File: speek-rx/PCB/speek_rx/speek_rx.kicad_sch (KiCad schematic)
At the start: 69 parts, among them CN1 PJ-320D, CN2 PJ-320D, J1 Conn_01x02, J3 Conn_01x06_Socket, J4 Conn_01x04, U1 ESP32-D0WD-V3, U2 W25Q32JVSSIQ_C179173, U3 CP2102N-A02-GQFN24R, U4 SPX1117M3-L-3-3/TR, U5 PCM5102APW, U6 TPA6132A2RTER, X1 XL2EL89CPI-111YLC-40M

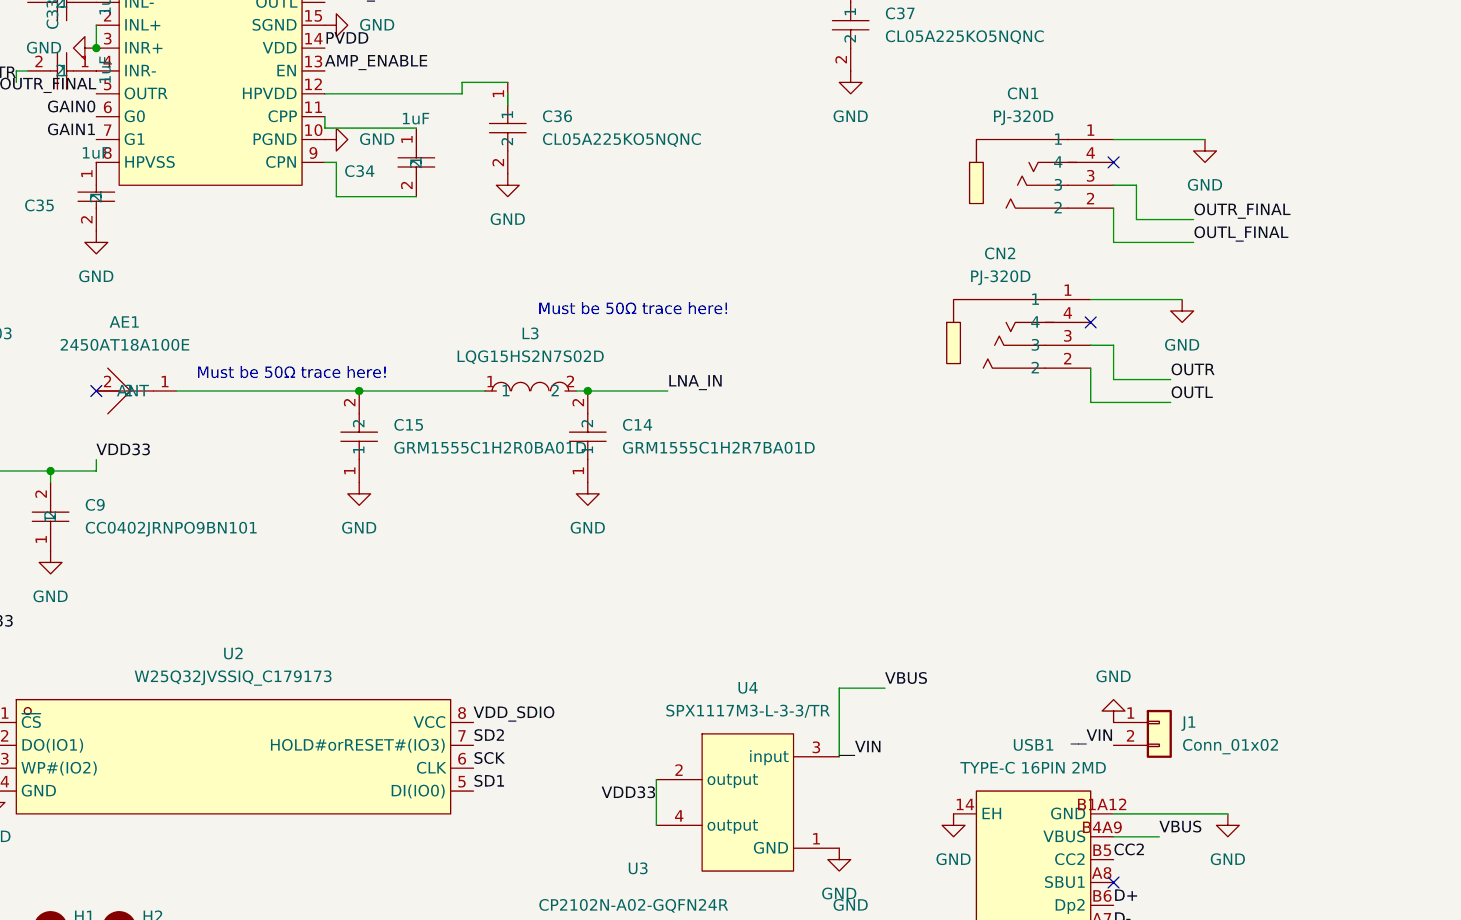
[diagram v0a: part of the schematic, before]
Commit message: JST and antenna
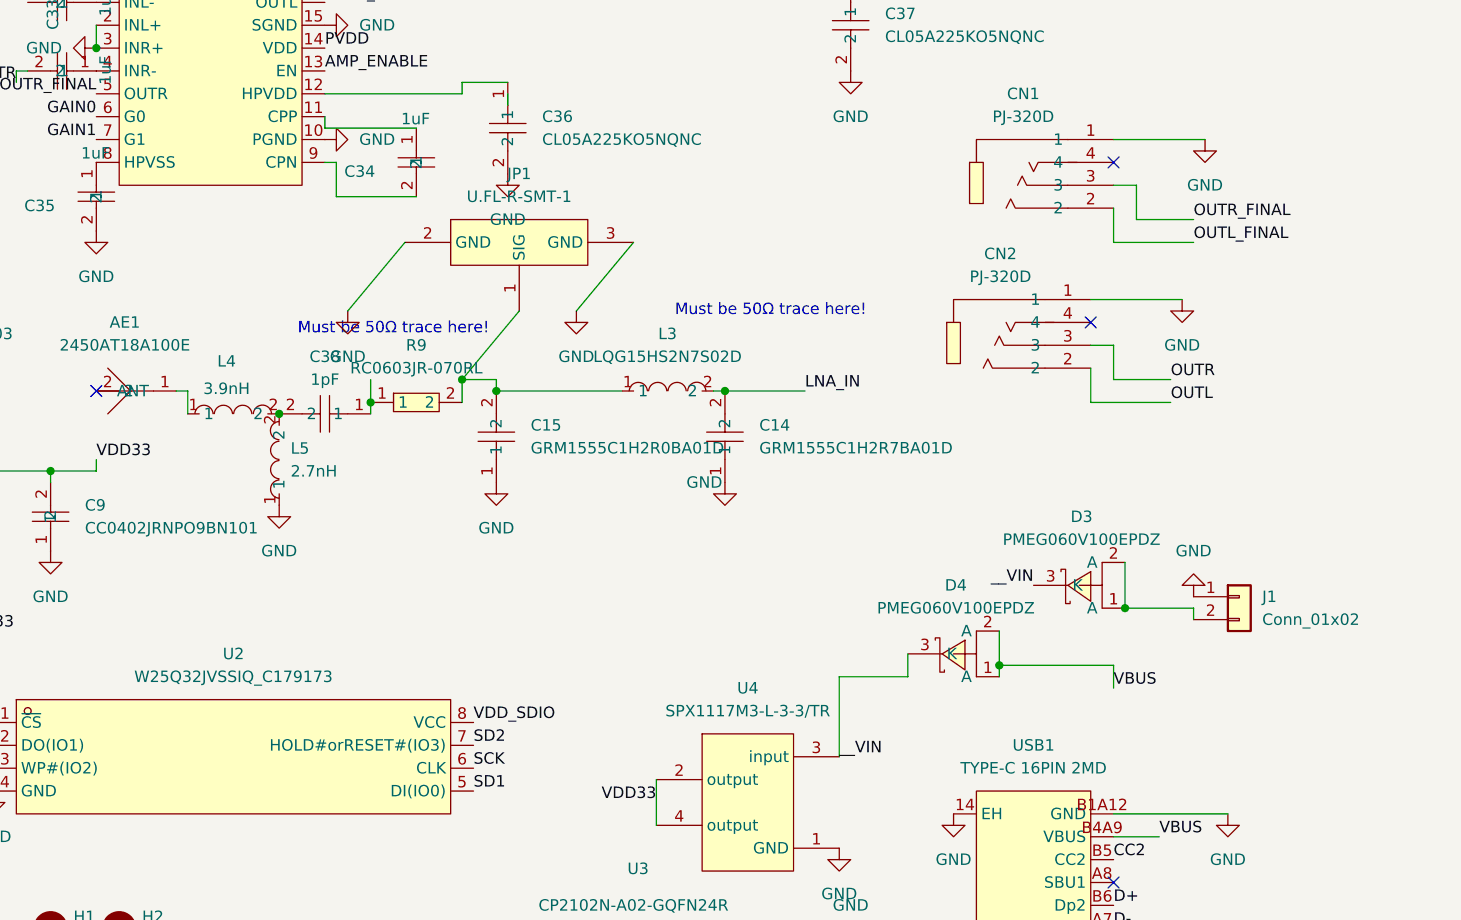
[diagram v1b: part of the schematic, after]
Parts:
- added C38: 1pF, easyeda2kicad:C0402, symbol lcsc:CC0402BRNPO9BN1R0
- added D3, D4: PMEG060V100EPDZ, easyeda2kicad:SOT1289_L5.8-W4.4-LS6.5-RD, symbol lcsc:PMEG060V100EPDZ
- added JP1: U.FL-R-SMT-1, easyeda2kicad:RF-SMD_FRF05002-JSS103M, symbol lcsc:U.FL-R-SMT-1
- added L4: 3.9nH, easyeda2kicad:IND-SMD_L1.0-W0.5-2, symbol lcsc:LQW15AN3N9B00D
- added L5: 2.7nH, easyeda2kicad:L0402, symbol lcsc:LQG15HS2N7S02D
- added R9: RC0603JR-070RL, easyeda2kicad:R0603, symbol lcsc:RC0603JR-070RL
- J1: footprint Connector_JST:JST_EH_S2B-EH_1x02_P2.50mm_Horizontal -> Connector_JST:JST_VH_B2P-VH-B_1x02_P3.96mm_Vertical
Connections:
- net GND: now also JP1.2 (GND), JP1.3 (GND), L5.1
- net VBUS: now also D4.1 (A), D4.2 (A); no longer J1.2 (Pin_2), J3.2 (Pin_2), U4.3 (input)
- net at C15.2, L3.1: now also JP1.1 (SIG), R9.2; no longer AE1.1 (ANT)
- new net: C38.1, R9.1
- new net: C38.2, L4.2, L5.2
- new net: D3.1 (A), D3.2 (A), J1.2 (Pin_2)
- new net: AE1.1 (ANT), L4.1
- new net __VIN: D3.3 (K), D4.3 (K), J3.2 (Pin_2), U4.3 (input)
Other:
- moved on the sheet: C14, C15, J1, L3

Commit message: speek rx schematic improvements
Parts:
- added Q1, Q2: SS8050-G, easyeda2kicad:SOT-23-3_L2.9-W1.5-P1.90-LS2.6-BR, symbol lcsc:SS8050-G_C3199946
- added R10, R11: 10k, easyeda2kicad:R0402, symbol lcsc:RC0402FR-0710KL
- R3: value RC0402FR-0710KL -> 10k
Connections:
- net CHIP_PU: now also Q1.3 (C); no longer J3.4 (Pin_4), U3.19 (RTS)
- net DTR: now also Q2.2 (E), R10.2; no longer BOOT1.2 (B), BOOT1.4 (D), C18.1, U1.23 (GPIO0)
- new net: Q2.1 (B), R11.1
- new net: Q1.1 (B), R10.1
- new net GPIO0: BOOT1.2 (B), BOOT1.4 (D), C18.1, Q2.3 (C), U1.23 (GPIO0)
- new net RTS: J3.4 (Pin_4), Q1.2 (E), R11.2, U3.19 (RTS)
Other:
- note added: "Antenna"
- note added: "Boot and EN buttons"
- note added: "DAC"
- note added: "ESP chip"
- note added: "Flash"
- note added: "Headphone amp"
- note added: "Output audio ports"
- note added: "Power / global"
- note added: "USB port"
- note added: "Uart converter"
- note removed: "No transistor circuit on purpose! It's just bloat, I have a good serial terminal"
- moved on the sheet: AE1, BOOT1, C1, C10, C11, C12, C13, C14, C15, C16, C17, C18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
